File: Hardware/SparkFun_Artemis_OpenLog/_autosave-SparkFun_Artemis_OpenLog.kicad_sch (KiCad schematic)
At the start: 92 parts, among them J11 Qwiic_RA, J14 CORTEX_JTAG, J2 Conn_01x02, J3 Conn_01x02, J4 CONN_06NO_SILK_NO_POP, J5 JST_2mm_LiPo, J6 MICRO-SD, J7 CONN_01PTH_NO_SILK_YES_STOP, J8 USB_C_Receptacle, Q2 DMG2305UX, U1 3.0V Supervisor, U10 CH340E, U2 MCP73831, U3 AP2112K-3.3, U4 3.3V, U5 BNO086, U8 ARTEMIS_MODULE, Y1 32.768kHz, Y3 32.768kHz

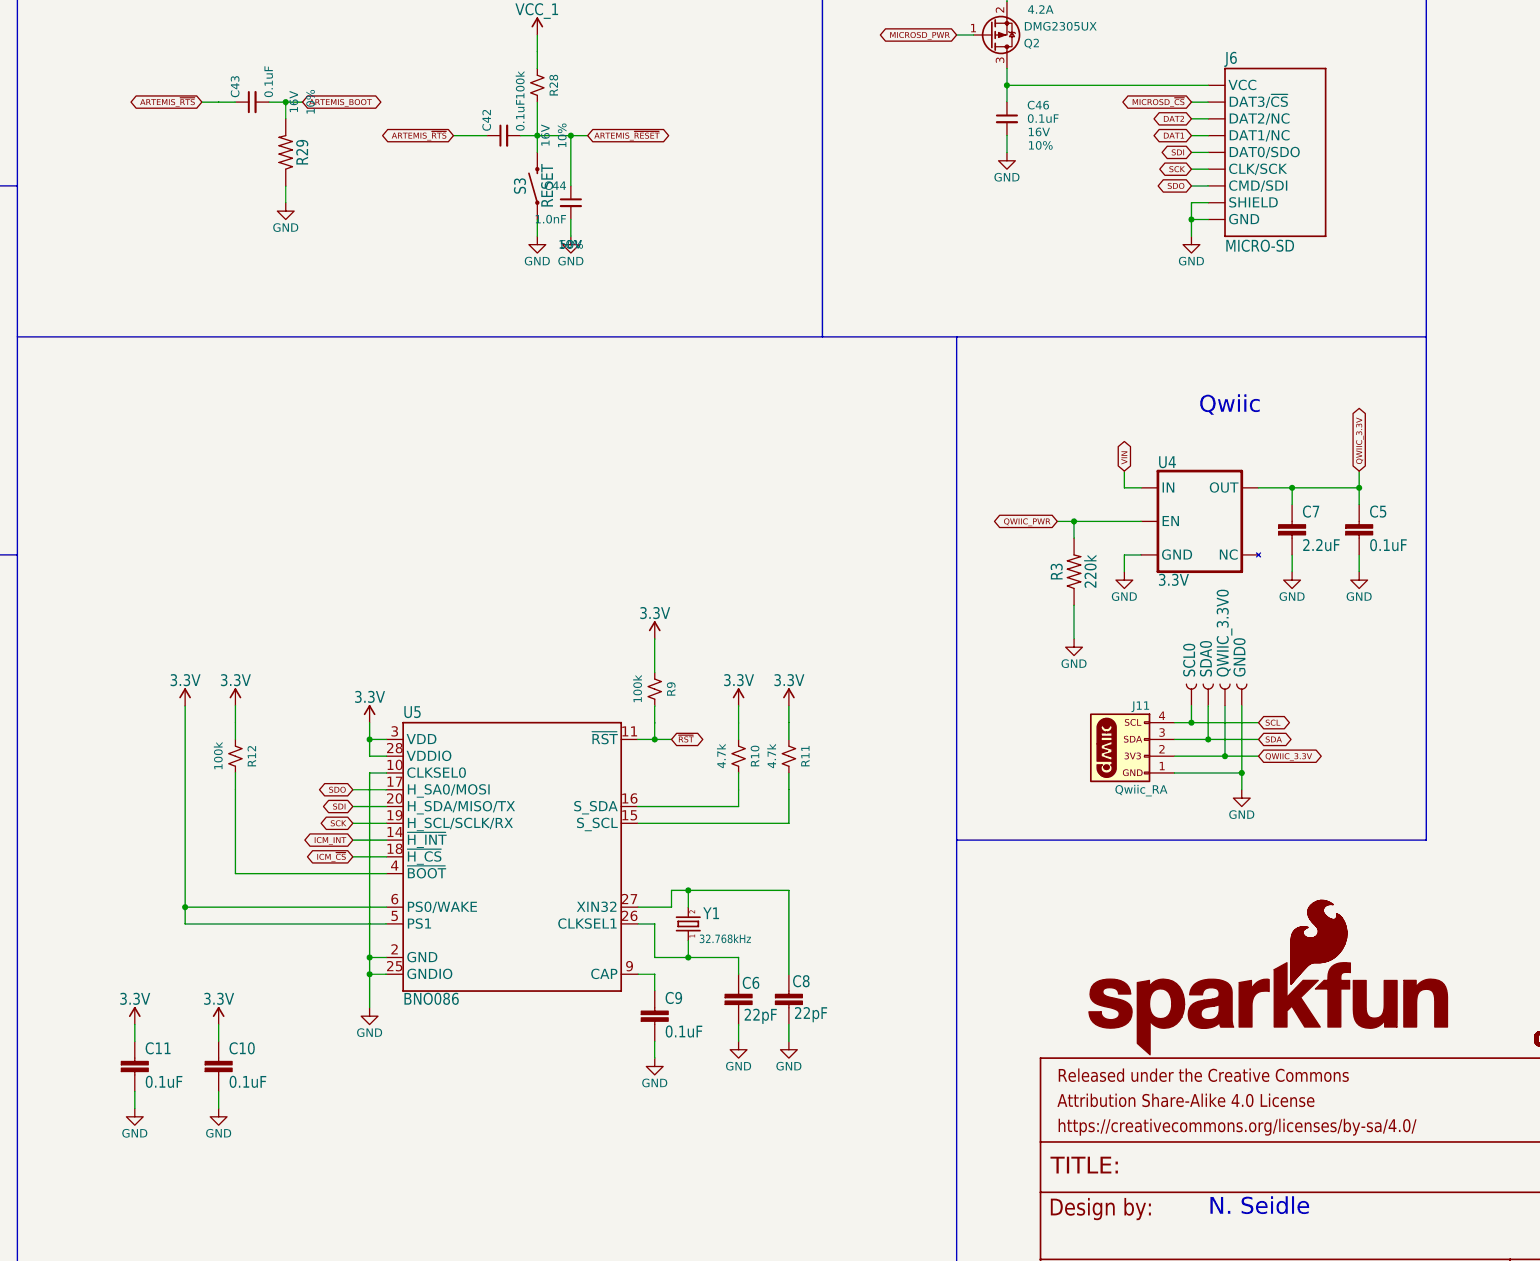
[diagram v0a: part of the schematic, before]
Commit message: Save spot
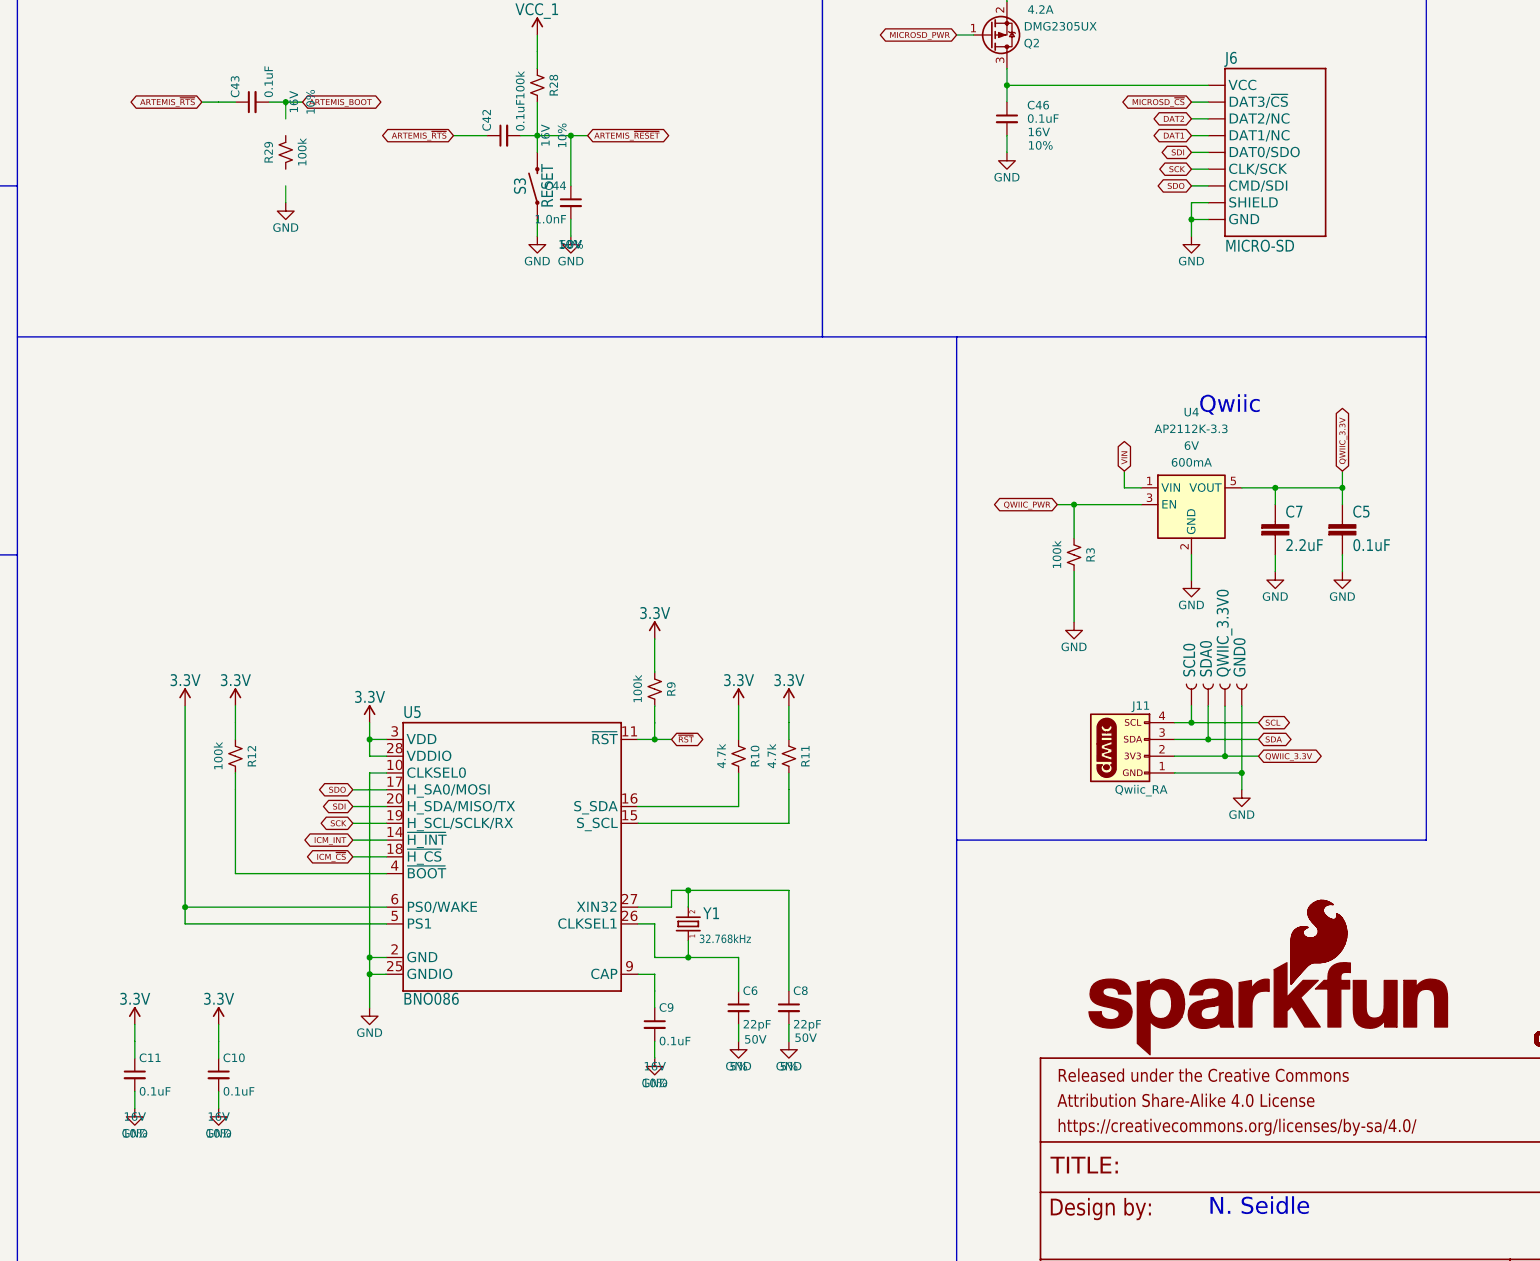
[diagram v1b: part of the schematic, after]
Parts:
- C10, C11, C9: footprint SparkFun_Artemis_OpenLog:0402 -> SparkFun-Capacitor:C_0402_1005Metric; symbol SparkFun_Artemis_OpenLog-eagle-import:0.1UF-0402-6.3V-10%-X7R -> SparkFun-Capacitor:0.1uF_0402_16V_10%; PROD_ID CAP-14993 -> CAP-25565; Tolerance (none) -> 10%; Voltage (none) -> 16V
- C6, C8: footprint SparkFun_Artemis_OpenLog:0402-TIGHT -> SparkFun-Capacitor:C_0402_1005Metric; symbol SparkFun_Artemis_OpenLog-eagle-import:22PF-0402T-16V-10% -> SparkFun-Capacitor:22pF_0402_50V_5%; PROD_ID CAP-14674 -> CAP-25012; Tolerance (none) -> 5%; Voltage (none) -> 50V
- R29: value 220KOHM-0402T-1/16W-1% -> 100k; footprint SparkFun_Artemis_OpenLog:0402-TIGHT -> SparkFun-Resistor:R_0402_1005Metric; symbol SparkFun_Artemis_OpenLog-eagle-import:220KOHM-0402T-1/16W-1% -> SparkFun-Resistor:100k_0402; PROD_ID RES-15094 -> RES-25013
- R3: value 220k -> 100k; footprint SparkFun_Artemis_OpenLog:0402-TIGHT -> SparkFun-Resistor:R_0402_1005Metric; symbol SparkFun_Artemis_OpenLog-eagle-import:220KOHM-0402T-1/16W-1% -> SparkFun-Resistor:100k_0402; PROD_ID RES-15094 -> RES-25013
- U4: value 3.3V -> AP2112K-3.3; footprint SparkFun_Artemis_OpenLog:SOT23-5 -> SparkFun-Semiconductor-Standard:SOT23-5; symbol SparkFun_Artemis_OpenLog-eagle-import:V_REG_AP2112K-3.3V -> SparkFun-Regulator:AP2112K-3.3; IMax (none) -> 600mA; Iq (none) -> 55µA; VMax (none) -> 6V
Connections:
- net ARTEMIS_BOOT: no longer R29.2
- net GND: no longer R29.1
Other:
- moved on the sheet: C5, C7
